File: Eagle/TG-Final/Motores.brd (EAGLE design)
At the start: 172.7 x 76.2 mm, 5 parts

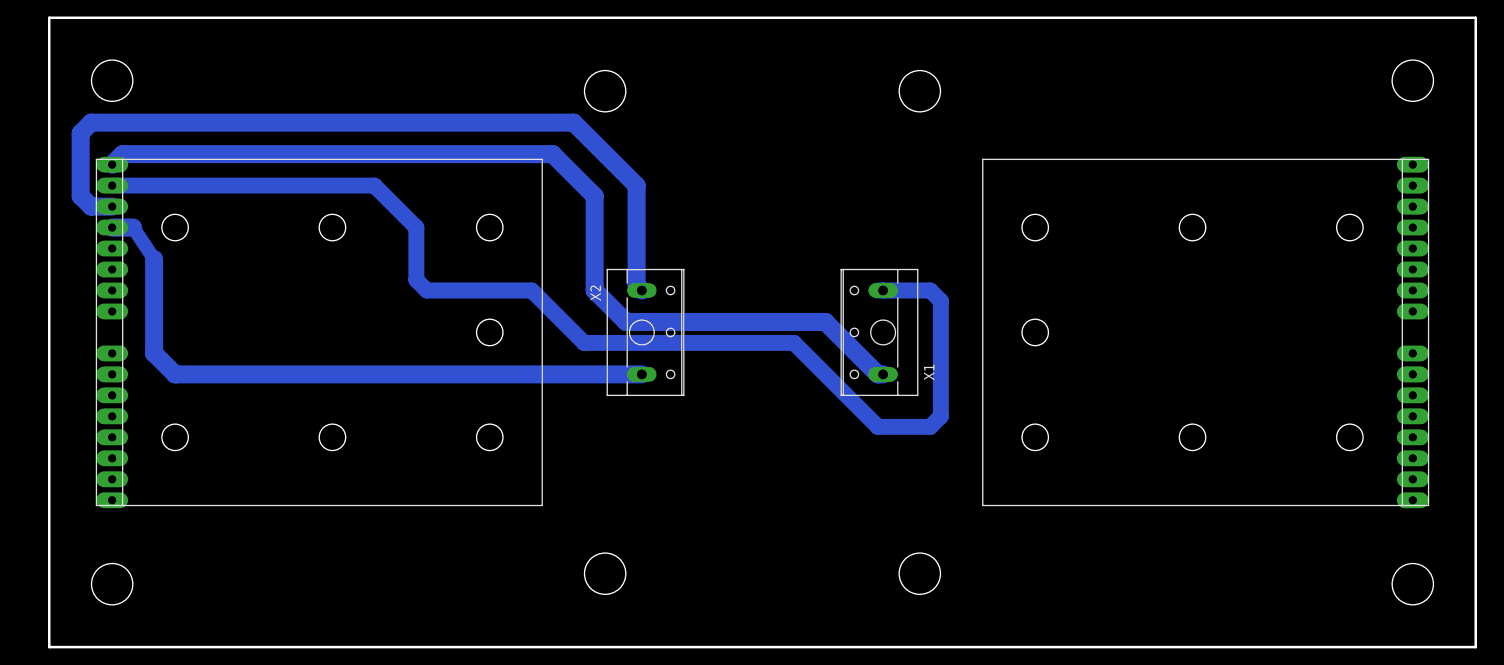
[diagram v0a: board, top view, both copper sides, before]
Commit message: Muchos Cambios a 2 dias de la denfesa
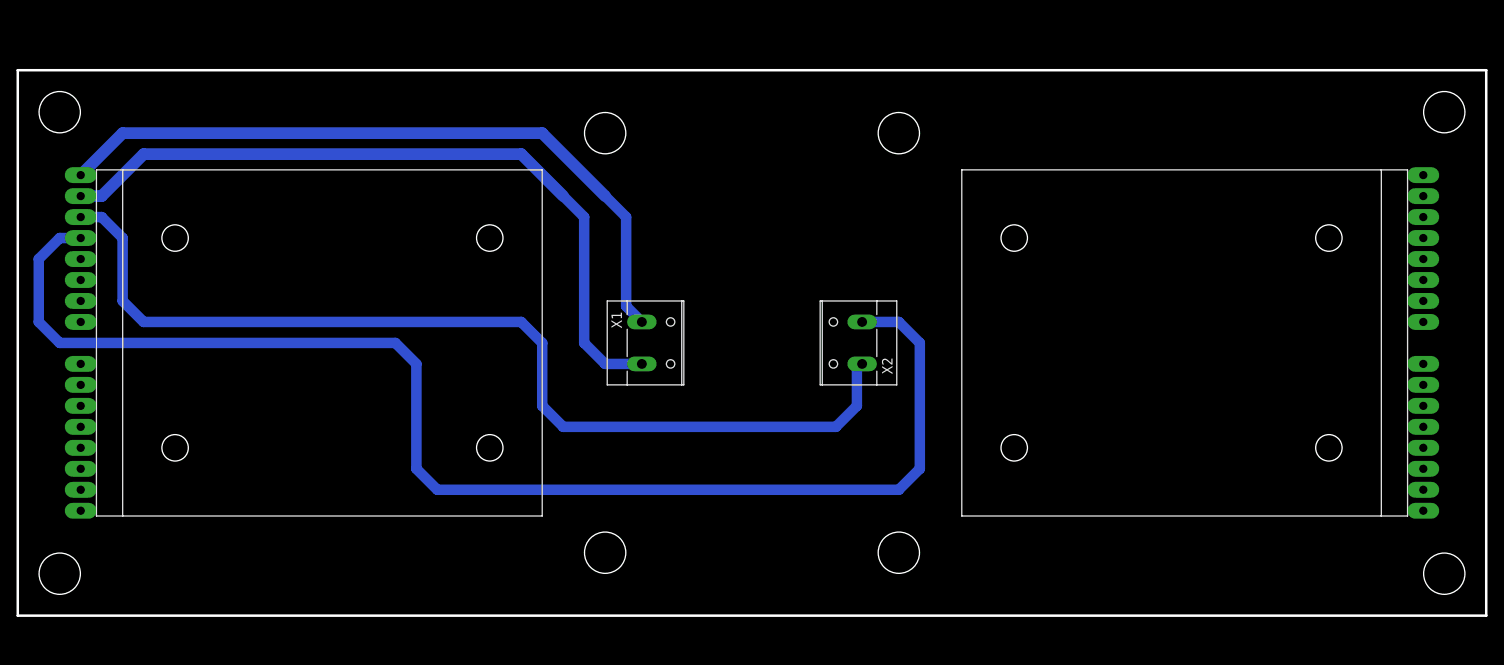
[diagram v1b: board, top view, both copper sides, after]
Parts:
- U$1: value BASEFINAL -> BASE-FINAL
- X1, X2: device con-wago-508:W237-2N -> con-wago-508:W237-132
- moved X1 28.0 mm to (-114.3, 38.1), turned to 270 degrees
- moved X2 25.4 mm to (-88.9, 38.1), turned to 90 degrees
- moved U$3 2.84 mm to (-50.8, 38.1)
- moved U$1 1.80 mm to (-101.6, 38.1)
- moved U$2 1.27 mm to (-152.4, 38.1)
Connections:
- net N$1: now also U$1.PIN01; no longer U$1.P$2
- net N$2: now also U$1.PIN02; no longer U$1.P$3
- net N$3: now also U$1.PIN03; no longer U$1.P$4
- net N$4: now also U$1.PIN00; no longer U$1.P$1
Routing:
- net N$3: track 78.7 -> 160.6 mm
- net N$1: track 138.8 -> 89.5 mm
- net N$4: track 111.6 -> 85.8 mm
- net N$2: track 95.9 -> 119.8 mm
- removed copper zone on layer 16, net N$5
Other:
- board size 172.7 x 76.2 mm -> 177.8 x 66 mm
